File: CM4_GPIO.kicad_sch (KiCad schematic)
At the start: 16 parts, among them IC5 74LVC1G07QSE-7, J3 2222, SW1 SW_Push, SW2 SW_Push, SW3 SW_Push

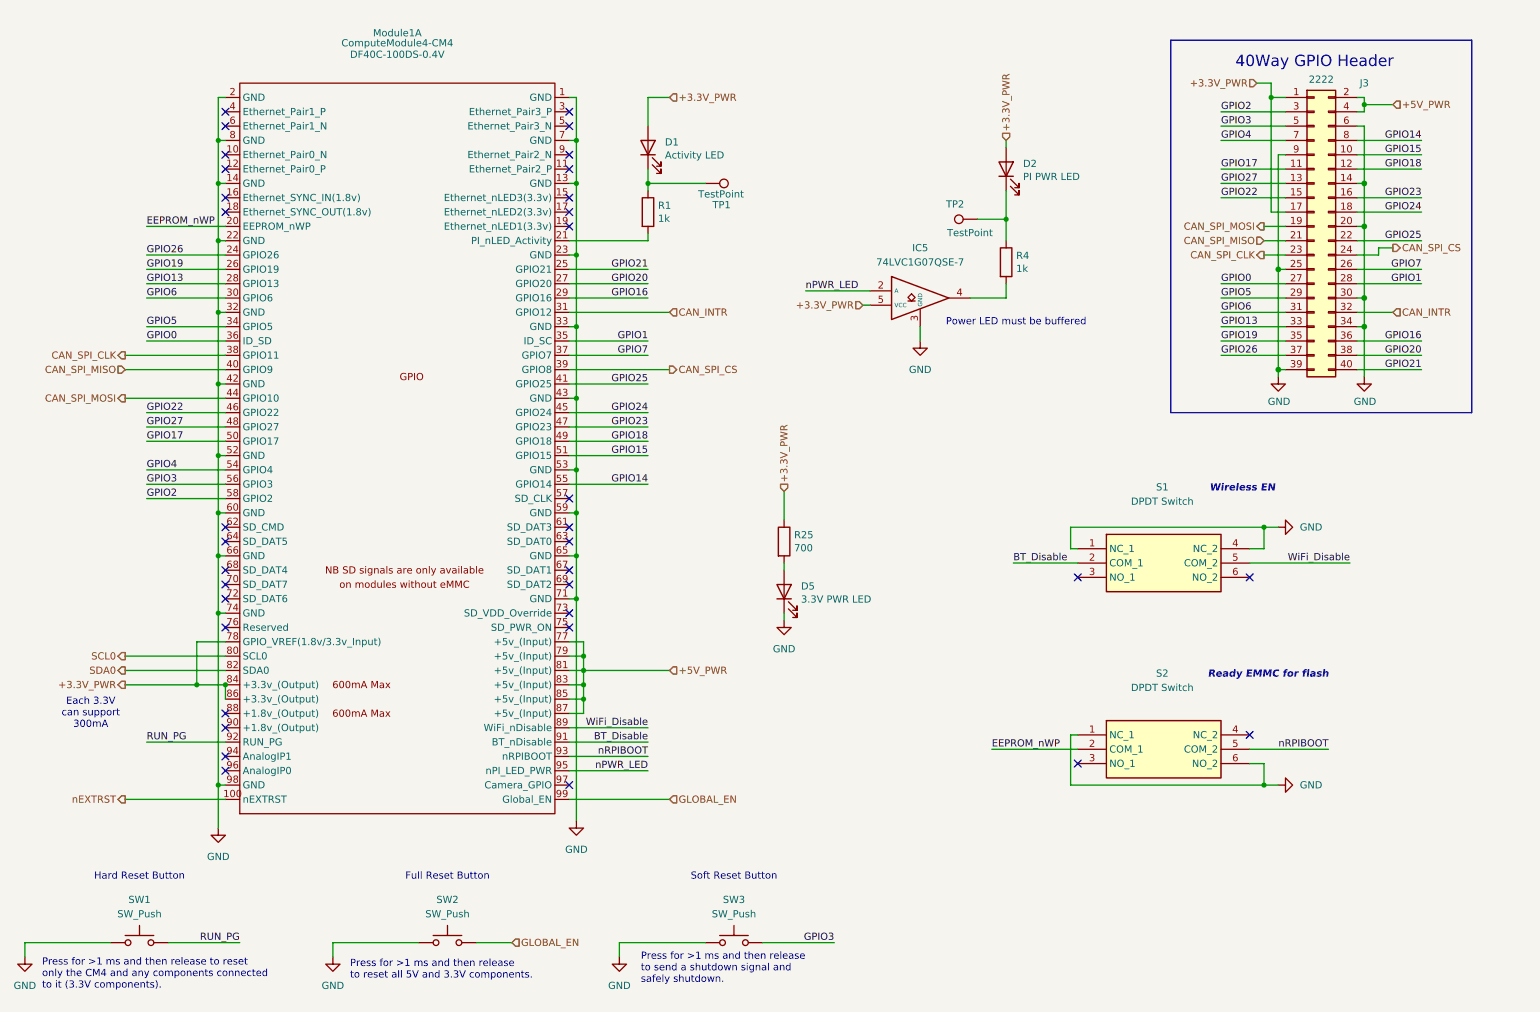
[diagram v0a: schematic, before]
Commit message: review committee changes implmented
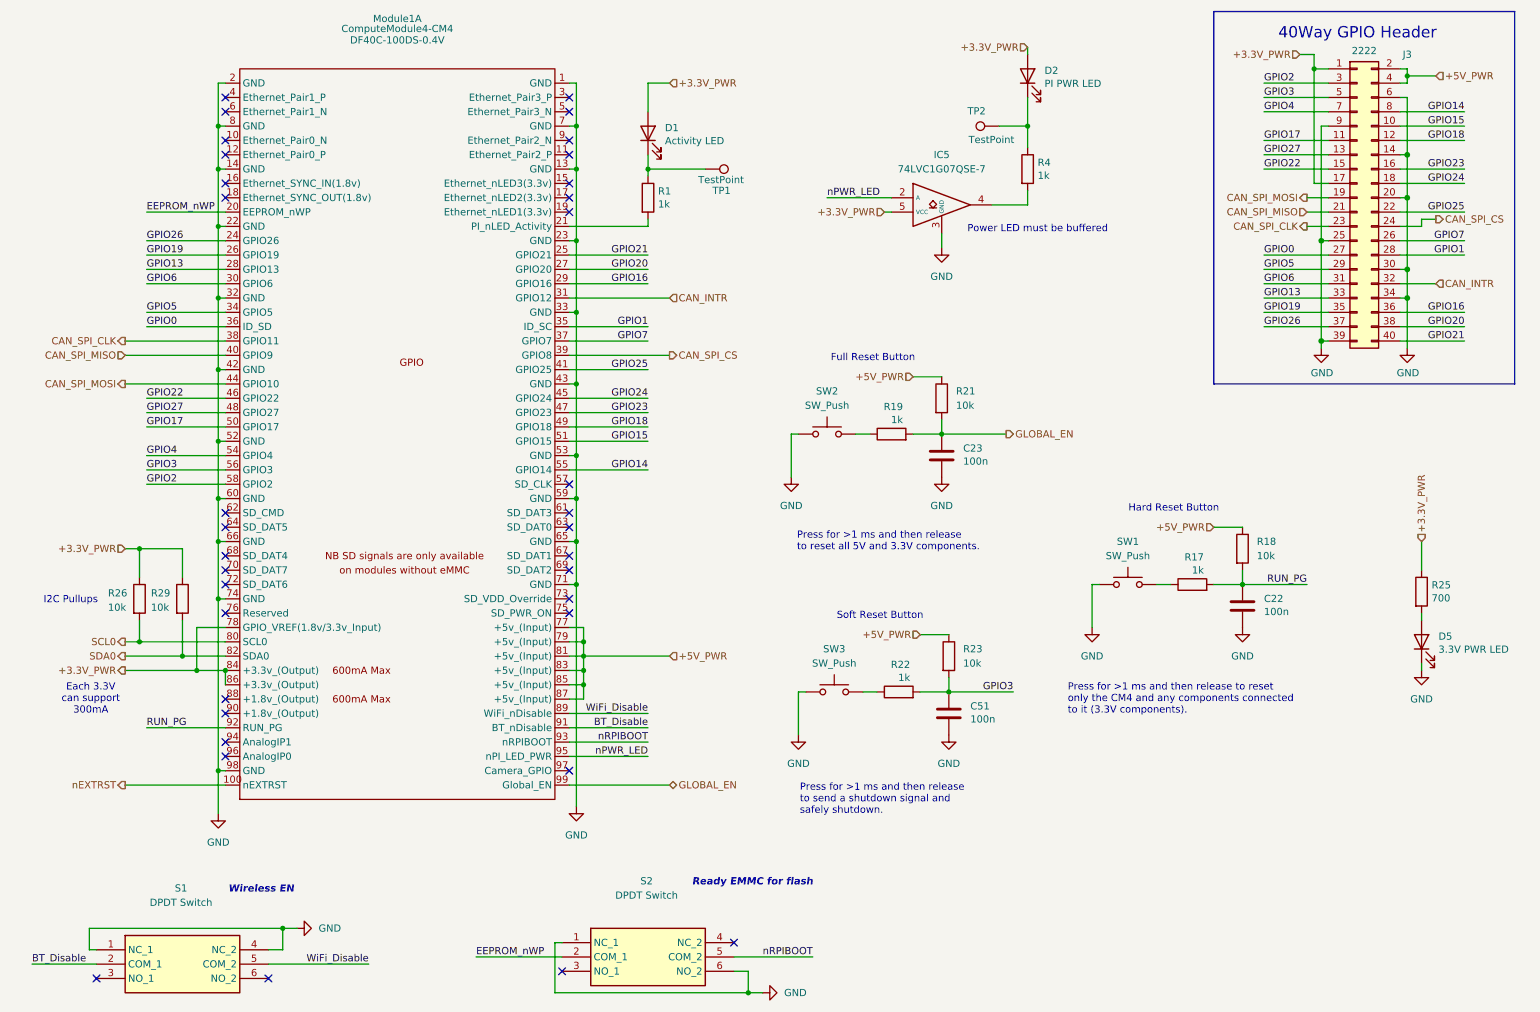
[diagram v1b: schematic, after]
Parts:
- added C22, C23, C51: 100n, Capacitor_SMD:C_0805_2012Metric, symbol Device:C
- added R17, R19, R22: 1k, Resistor_SMD:R_0805_2012Metric, symbol Device:R
- added R18, R21, R23, R26, R29: 10k, Resistor_SMD:R_0805_2012Metric, symbol Device:R
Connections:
- net +3.3V_PWR: now also R26.1, R29.1
- net +5V_PWR: now also R18.1, R21.1, R23.1
- net GLOBAL_EN: now also C23.1, R19.2, R21.2; no longer SW2.2
- net GND: now also C22.2, C23.2, C51.2
- net GPIO3: now also C51.1, R22.2, R23.2; no longer SW3.2
- net RUN_PG: now also C22.1, R17.2, R18.2; no longer SW1.2
- net SCL0: now also R26.2
- net SDA0: now also R29.2
- new net: R17.1, SW1.2
- new net: R19.1, SW2.2
- new net: R22.1, SW3.2
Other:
- note added: "I2C Pullups"
- moved on the sheet: D1, D2, D5, IC5, J3, Module1A, R1, R25, R4, S1, S2, SW1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
